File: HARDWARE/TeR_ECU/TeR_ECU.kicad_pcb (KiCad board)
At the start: 4 copper layers, 42 parts, among them IC1 MX34040NF2, J2 RJ45_Shielded, J3 RJ45_Shielded, J4 RJ45_Shielded, Q1 ZXMN3F30FH, Q2 ZXMN3F30FH, U2 SN65HVD230, U3 SN65HVD230, U4 LM1117MP-3.3, U5 TSR_1-2450, U7 HDSP-A153, U8 NUCLEO144-F746ZG

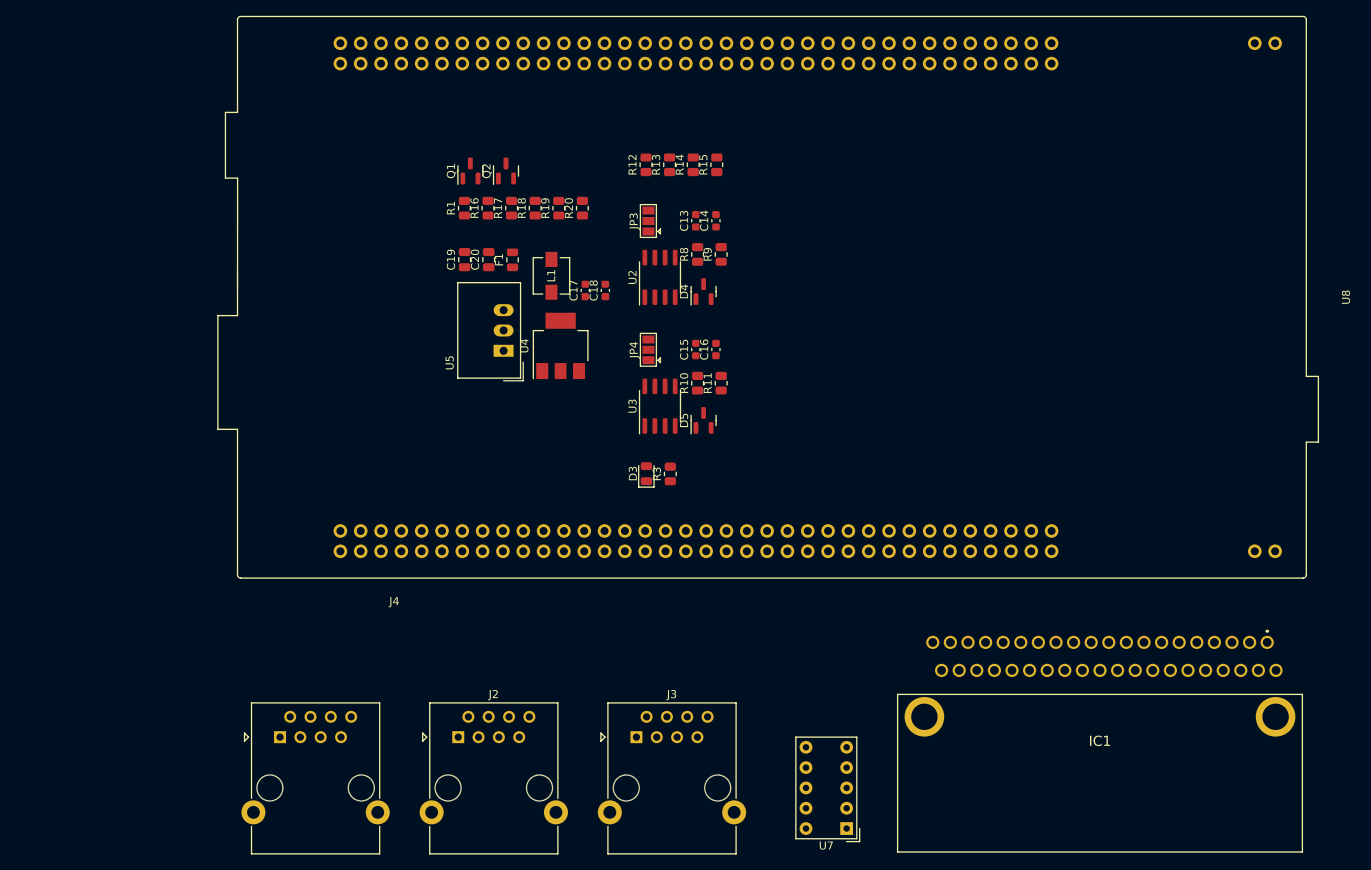
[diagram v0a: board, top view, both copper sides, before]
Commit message: Empezando Layout
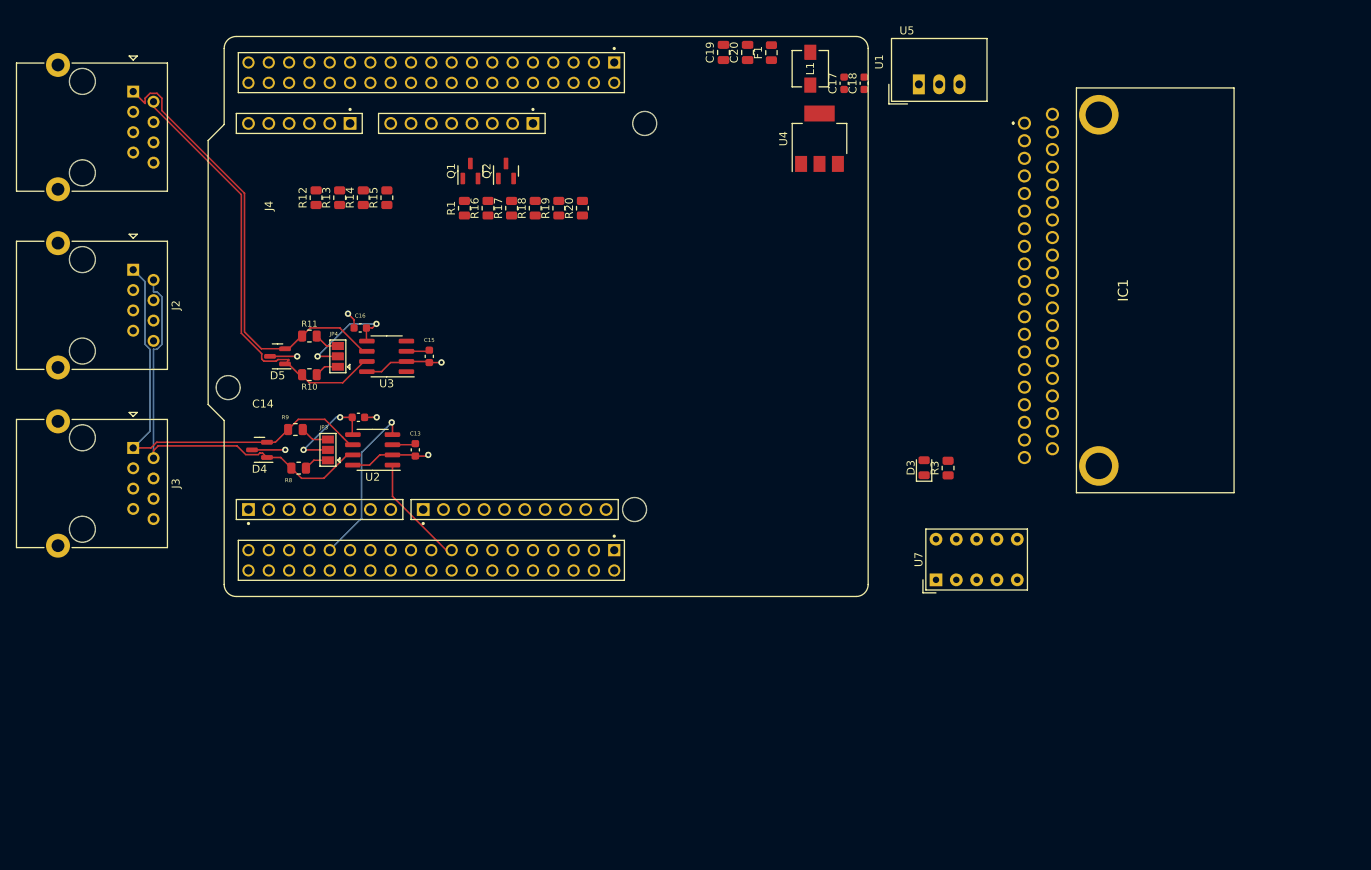
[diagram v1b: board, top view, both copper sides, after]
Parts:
- removed U8: NUCLEO144-F746ZG, Module:ST_Morpho_Connector_144_STLink
- added U1: NUCLEO-F446RE, Nucleo-F446RE:MODULE_NUCLEO-F446RE, F.Cu at (111.3, 79.0)
- moved J4 82.8 mm to (60.6, 50.8), turned to -90 degrees
- moved J3 72.6 mm to (60.6, 95.4), turned to -90 degrees
- moved J2 71.2 mm to (60.6, 73.1), turned to -90 degrees
- moved U5 61.7 mm to (158.9, 49.9), turned to 0 degrees
- moved D4 58.9 mm to (76.4, 95.6), turned to 180 degrees
- moved R9 57.5 mm to (80.9, 93.1), turned to 180 degrees
- moved R8 56.6 mm to (81.3, 97.9), turned to 0 degrees
- moved IC1 56.4 mm to (184.4, 75.7), turned to 90 degrees
- moved D5 53.9 mm to (78.7, 83.9), turned to 180 degrees
- moved R11 51.8 mm to (82.7, 81.4), turned to 180 degrees
- moved C14 51.0 mm to (88.8, 91.6), turned to 0 degrees
- moved JP3 49.2 mm to (85.0, 95.6)
- moved R10 48.5 mm to (82.7, 86.2), turned to 0 degrees
- moved C13 45.3 mm to (95.9, 95.6)
- moved C16 44.5 mm to (89.0, 80.4), turned to 180 degrees
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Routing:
- net /CAN_POWERTRAIN/CAN-: track 0.00 -> 57.3 mm
- net /CAN_POWERTRAIN/CAN+: track 0.00 -> 54.4 mm
- net /CAN_MAIN/CAN-: track 0.00 -> 54.3 mm
- net /CAN_MAIN/CAN+: track 0.00 -> 52.8 mm
- net GND: track 0.00 -> 31.2 mm, vias 0 -> 6
- net /CAN_MAIN/CAN_RX: track 0.00 -> 20.7 mm, vias 0 -> 1
- net /CAN_POWERTRAIN/VREF: track 0.00 -> 14.7 mm, vias 0 -> 2
- net /CAN_MAIN/CAN_TX: track 0.00 -> 14.1 mm
- net /CAN_MAIN/VREF: track 0.00 -> 13.0 mm, vias 0 -> 2
- net +3.3V: track 0.00 -> 5.83 mm
- net Net-(JP3-B): track 0.00 -> 3.67 mm
- net Net-(JP4-B): track 0.00 -> 3.16 mm
- net Net-(JP3-A): track 0.00 -> 3.16 mm
- net Net-(JP4-A): track 0.00 -> 3.05 mm
- added copper zone on In1.Cu, net GND
